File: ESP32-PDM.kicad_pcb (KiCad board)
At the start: 2 copper layers, 38.4 x 55.4 mm, 21 parts, among them J1 Conn_02x04_Top_Bottom, J2 Conn_02x06_Top_Bottom, U1 TPS1H100AQPWPRQ1, U2 TPS1H100AQPWPRQ1, U3 TPS1H100AQPWPRQ1, U4 TPS1H100AQPWPRQ1

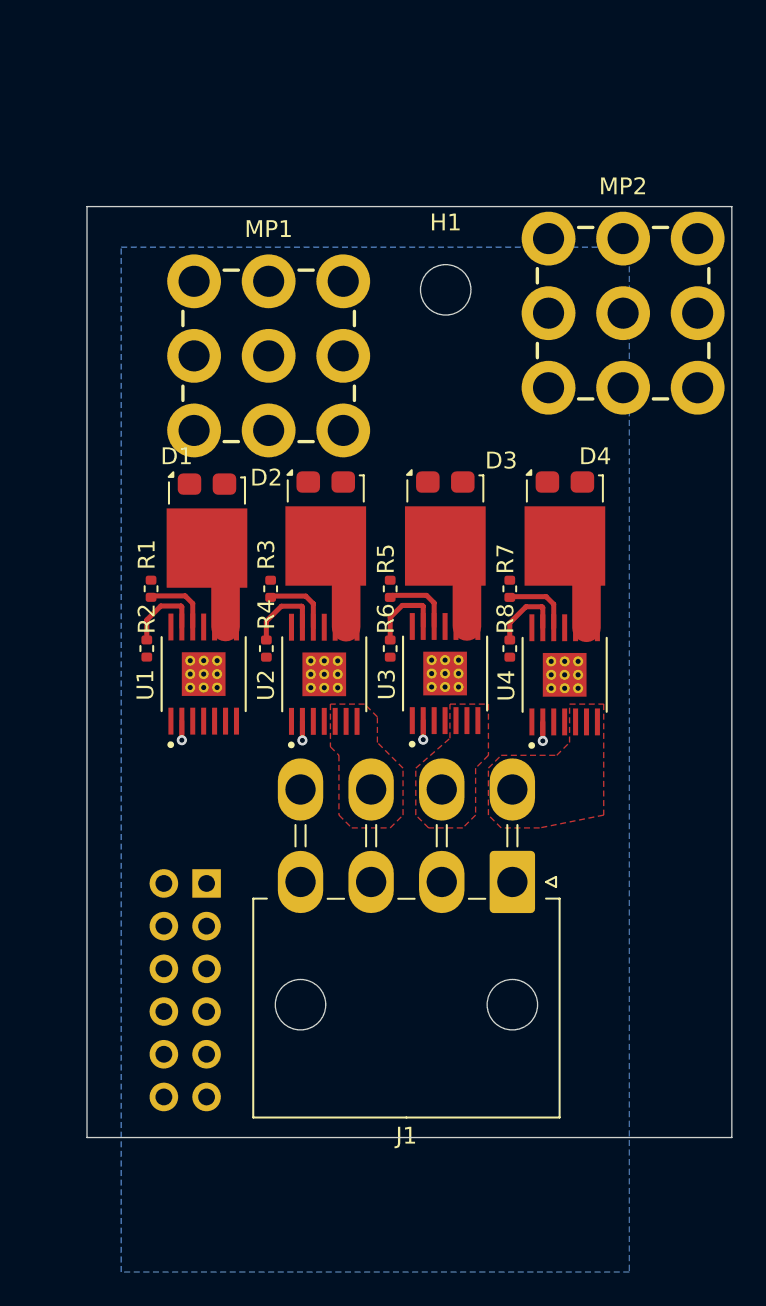
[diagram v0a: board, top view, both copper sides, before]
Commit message: PCB first version
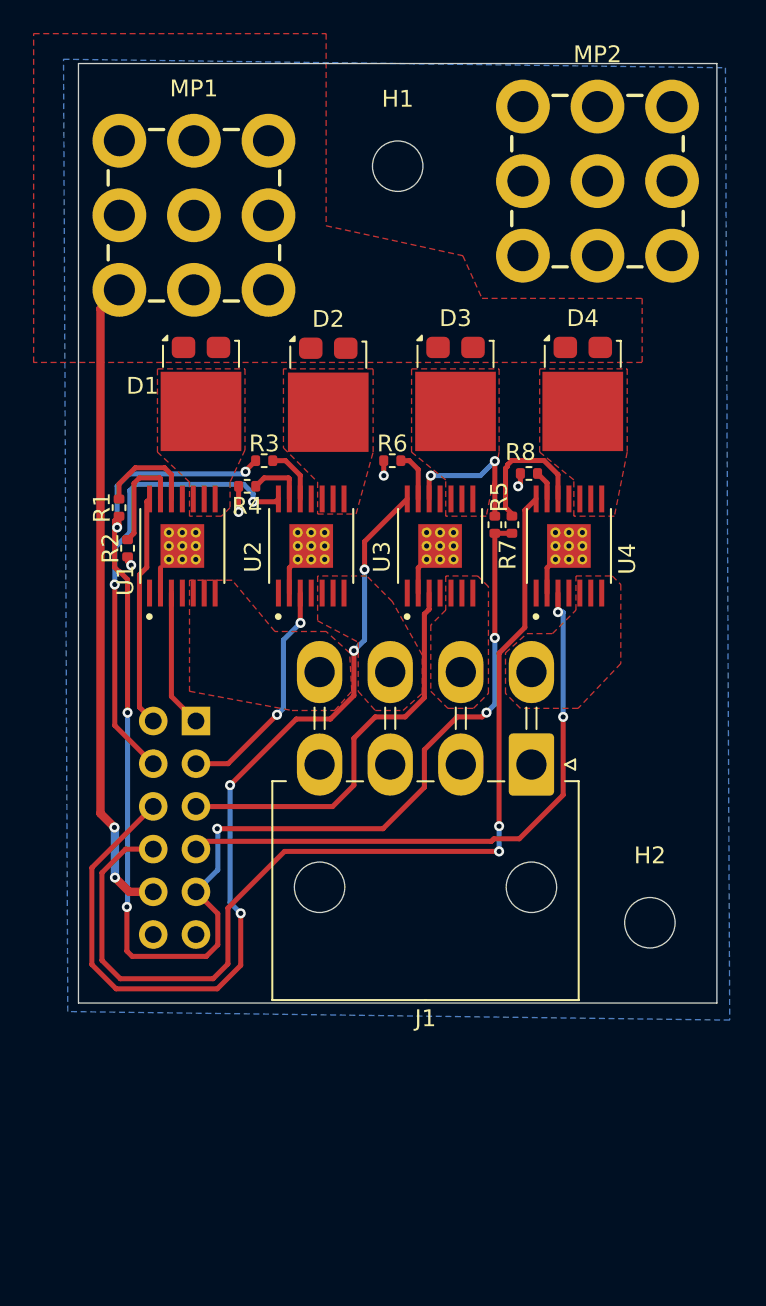
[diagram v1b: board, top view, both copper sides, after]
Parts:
- added H2: MountingHole, MountingHole:MountingHole_3mm, F.Cu at (130.0, 92.0)
- J1: value Conn_02x04_Top_Bottom -> 5569-08A2-210
- moved R6 11.2 mm to (114.7, 64.5), turned to 180 degrees
- moved R8 10.5 mm to (122.8, 65.3), turned to 180 degrees
- moved R4 9.72 mm to (106.0, 66.0), turned to 180 degrees
- moved J2 9.68 mm to (103.0, 80.0)
- moved MP1 9.47 mm to (102.9, 49.9)
- moved D1 8.14 mm to (103.3, 60.5)
- moved D4 8.08 mm to (126.0, 60.5)
- moved D3 8.03 mm to (118.4, 60.5)
- moved MP2 8.00 mm to (126.9, 47.9)
- moved D2 7.96 mm to (110.9, 60.6)
- moved H1 7.89 mm to (115.0, 47.0)
- moved U1 7.73 mm to (102.2, 69.6)
- moved U2 7.67 mm to (109.9, 69.6)
- moved U4 7.67 mm to (125.2, 69.6)
- moved R3 7.63 mm to (107.1, 64.5), turned to 180 degrees
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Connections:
- net /SUPPLY renamed VS
- net Net-(J1-Pin_5) renamed /OUT4
- net Net-(J1-Pin_6) renamed /OUT3
- net Net-(J1-Pin_7) renamed /OUT2
- net Net-(J1-Pin_8) renamed /OUT1
- net Net-(J2-Pin_1) renamed /IN1
- net Net-(J2-Pin_2) renamed /DIAG1
- net Net-(J2-Pin_3) renamed /IN2
- net Net-(J2-Pin_4) renamed /DIAG2
- net Net-(J2-Pin_5) renamed /IN3
- net Net-(J2-Pin_6) renamed /DIAG3
- net Net-(J2-Pin_7) renamed /IN4
- net Net-(J2-Pin_8) renamed /DIAG4
- J2 pad 12: unconnected-(J2-Pin_12-Pad12) -> GND
- R1 pad 1: +3.3V -> Net-(U1-DIAG_EN)
- R1 pad 2: Net-(U1-DIAG_EN) -> +3.3V
- R2 pad 1: GND -> Net-(U1-CL)
- R2 pad 2: Net-(U1-CL) -> GND
- R3 pad 1: +3.3V -> Net-(U2-DIAG_EN)
- R3 pad 2: Net-(U2-DIAG_EN) -> +3.3V
- R5 pad 1: +3.3V -> Net-(U3-DIAG_EN)
- R5 pad 2: Net-(U3-DIAG_EN) -> +3.3V
- R7 pad 1: +3.3V -> Net-(U4-DIAG_EN)
- R7 pad 2: Net-(U4-DIAG_EN) -> +3.3V
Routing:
- net +3.3V: track 0.00 -> 84.3 mm, vias 0 -> 7
- net /DIAG4: track 0.00 -> 59.9 mm, vias 0 -> 2
- net /DIAG3: track 0.00 -> 54.5 mm, vias 0 -> 4
- net VS: track 0.00 -> 38.4 mm, vias 0 -> 2
- net /IN4: track 0.00 -> 35.5 mm, vias 0 -> 2
- net /DIAG2: track 0.00 -> 27.4 mm, vias 0 -> 2
- net /IN3: track 0.00 -> 24.3 mm
- net /IN2: track 0.00 -> 13.9 mm, vias 0 -> 2
- net /DIAG1: track 0.00 -> 13.8 mm
- net /IN1: track 0.00 -> 8.21 mm
- net GND: track 4.53 -> 11.9 mm
- net Net-(D1-K): track 5.53 -> 0.00 mm
- net Net-(D4-K): track 5.14 -> 0.00 mm
- net Net-(D2-K): track 5.08 -> 0.00 mm
- net Net-(D3-K): track 5.07 -> 0.00 mm
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- added copper zone on F.Cu, net /OUT1
- added copper zone on F.Cu, net Net-(D1-K)
- added copper zone on F.Cu, net Net-(D2-K)
- added copper zone on F.Cu, net Net-(D3-K)
- added copper zone on F.Cu, net Net-(D4-K)
- added copper zone on F.Cu, net VS
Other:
- board size 38.4 x 55.4 mm -> 38 x 55.9 mm
